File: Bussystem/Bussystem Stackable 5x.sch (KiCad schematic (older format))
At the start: 11 parts, among them J1 PCIE-098-02-X-D-TH, J2 PCIE-098-02-X-D-TH, J3 PCIE-098-02-X-D-TH, J4 PCIE-098-02-X-D-TH, J5 PCIE-098-02-X-D-TH, J6 PCIE-098-02-X-D-EMS2-BG, J7 8x Edge conn

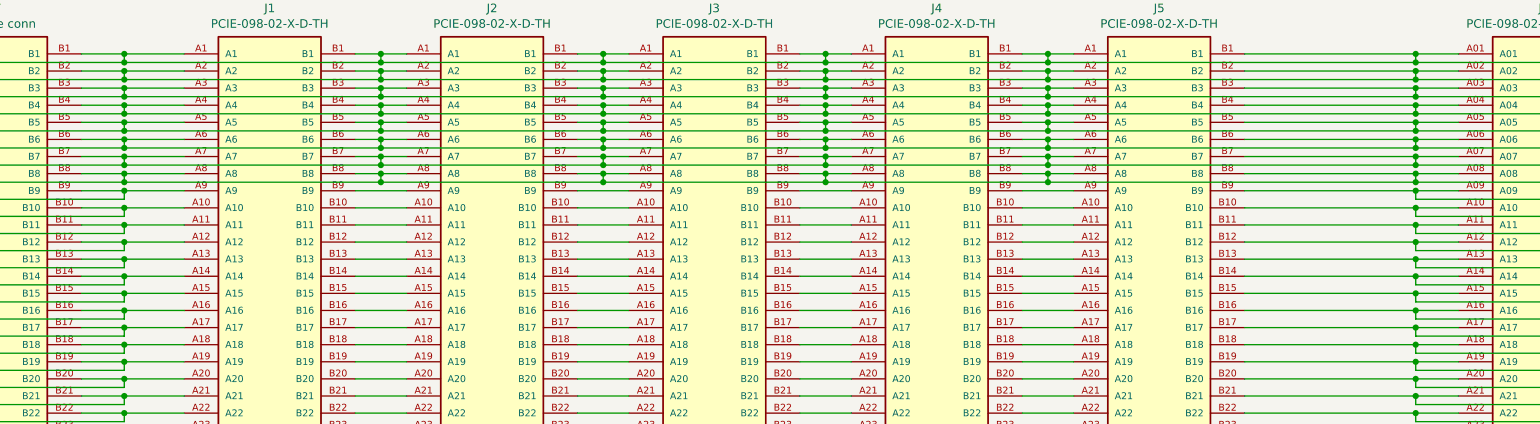
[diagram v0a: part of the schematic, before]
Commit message: first 10x Bus baseplate design. Still needs some redesign
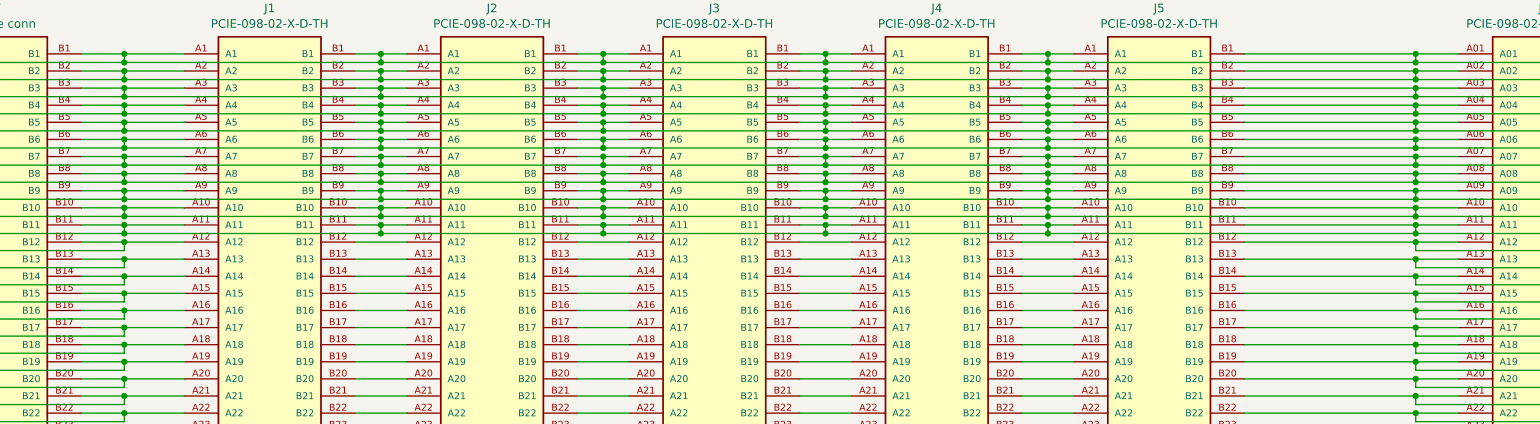
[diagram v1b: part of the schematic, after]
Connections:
- net at J1.A10, J7.A10, J7.B10: now also J1.B10, J2.A10, J2.B10, J3.A10, J3.B10, J4.A10, J4.B10, J5.A10, J5.B10, J6.A10, J6.B10
- net at J1.A11, J7.A11, J7.B11: now also J1.B11, J2.A11, J2.B11, J3.A11, J3.B11, J4.A11, J4.B11, J5.A11, J5.B11, J6.A11, J6.B11
- net at J1.A9, J7.A9, J7.B9: now also J1.B9, J2.A9, J2.B9, J3.A9, J3.B9, J4.A9, J4.B9, J5.A9, J5.B9, J6.A09, J6.B09
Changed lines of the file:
@@
 	3400 1750 3550 1750
 Wire Wire Line
-	3700 1850 3400 1850
-Wire Wire Line
-	3400 1950 3700 1950
-Wire Wire Line
-	3700 2050 3400 2050
+	3700 1850 3550 1850
+Wire Wire Line
+	3400 1950 3550 1950
+Wire Wire Line
+	3700 2050 3550 2050
 Wire Wire Line
 	3400 2150 3700 2150
@@
 	4700 1750 4850 1750
 Wire Wire Line
-	5000 1850 4700 1850
-Wire Wire Line
-	4700 1950 5000 1950
-Wire Wire Line
-	5000 2050 4700 2050
+	5000 1850 4850 1850
+Wire Wire Line
+	4700 1950 4850 1950
+Wire Wire Line
+	5000 2050 4850 2050
 Wire Wire Line
 	4700 2150 5000 2150
@@
 	6000 1750 6150 1750
 Wire Wire Line
-	6300 1850 6000 1850
-Wire Wire Line
-	6000 1950 6300 1950
-Wire Wire Line
-	6300 2050 6000 2050
+	6300 1850 6150 1850
+Wire Wire Line
+	6000 1950 6150 1950
+Wire Wire Line
+	6300 2050 6150 2050
 Wire Wire Line
 	6000 2150 6300 2150
@@
 	7300 1750 7450 1750
 Wire Wire Line
-	7600 1850 7300 1850
-Wire Wire Line
-	7300 1950 7600 1950
-Wire Wire Line
-	7600 2050 7300 2050
+	7600 1850 7450 1850
+Wire Wire Line
+	7300 1950 7450 1950
+Wire Wire Line
+	7600 2050 7450 2050
 Wire Wire Line
 	7300 2150 7600 2150
@@
 Connection ~ 7450 1800
 Connection ~ 9600 1800
+Wire Wire Line
+	2050 1900 3550 1900
+Connection ~ 2050 1900
+Connection ~ 9600 1900
+Wire Wire Line
+	7450 1900 7450 1850
+Connection ~ 7450 1900
+Wire Wire Line
+	7450 1900 9600 1900
+Connection ~ 7450 1850
+Wire Wire Line
+	7450 1850 7300 1850
+Wire Wire Line
+	6150 1900 6150 1850
+Connection ~ 6150 1900
+Wire Wire Line
+	6150 1900 7450 1900
+Connection ~ 6150 1850
+Wire Wire Line
+	6150 1850 6000 1850
+Wire Wire Line
+	3550 1900 3550 1850
+Connection ~ 3550 1900
+Wire Wire Line
+	3550 1900 4850 1900
+Connection ~ 3550 1850
+Wire Wire Line
+	3550 1850 3400 1850
+Wire Wire Line
+	4850 1900 4850 1850
+Connection ~ 4850 1900
+Wire Wire Line
+	4850 1900 6150 1900
+Connection ~ 4850 1850
+Wire Wire Line
+	4850 1850 4700 1850
+Wire Wire Line
+	2050 2000 3550 2000
+Wire Wire Line
+	3550 2000 3550 1950
+Connection ~ 2050 2000
+Connection ~ 3550 1950
+Wire Wire Line
+	3550 1950 3700 1950
+Wire Wire Line
+	3550 2000 4850 2000
+Connection ~ 3550 2000
+Connection ~ 9600 2000
+Wire Wire Line
+	7450 2000 7450 1950
+Connection ~ 7450 2000
+Wire Wire Line
+	7450 2000 9600 2000
+Connection ~ 7450 1950
+Wire Wire Line
+	7450 1950 7600 1950
+Wire Wire Line
+	6150 2000 6150 1950
+Connection ~ 6150 2000
+Wire Wire Line
+	6150 2000 7450 2000
+Connection ~ 6150 1950
+Wire Wire Line
+	6150 1950 6300 1950
+Wire Wire Line
+	4850 2000 4850 1950
+Connection ~ 4850 2000
+Wire Wire Line
+	4850 2000 6150 2000
+Connection ~ 4850 1950
+Wire Wire Line
+	4850 1950 5000 1950
+Wire Wire Line
+	2050 2100 3550 2100
+Connection ~ 2050 2100
+Connection ~ 9600 2100
+Wire Wire Line
+	7450 2100 7450 2050
+Connection ~ 7450 2100
+Wire Wire Line
+	7450 2100 9600 2100
+Connection ~ 7450 2050
+Wire Wire Line
+	7450 2050 7300 2050
+Wire Wire Line
+	6150 2100 6150 2050
+Connection ~ 6150 2100
+Wire Wire Line
+	6150 2100 7450 2100
+Connection ~ 6150 2050
+Wire Wire Line
+	6150 2050 6000 2050
+Wire Wire Line
+	3550 2100 3550 2050
+Connection ~ 3550 2100
+Wire Wire Line
+	3550 2100 4850 2100
+Connection ~ 3550 2050
+Wire Wire Line
+	3550 2050 3400 2050
+Wire Wire Line
+	4850 2100 4850 2050
+Connection ~ 4850 2100
+Wire Wire Line
+	4850 2100 6150 2100
+Connection ~ 4850 2050
+Wire Wire Line
+	4850 2050 4700 2050
 $EndSCHEMATC
